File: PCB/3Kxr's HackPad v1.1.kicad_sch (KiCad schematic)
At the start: 8 parts, among them SW1 SW_Push, SW2 SW_Push, SW3 SW_Push, SW4 SW_Push, SW8 RotaryEncoder_Switch, U1 XIAO-RP2040-DIP

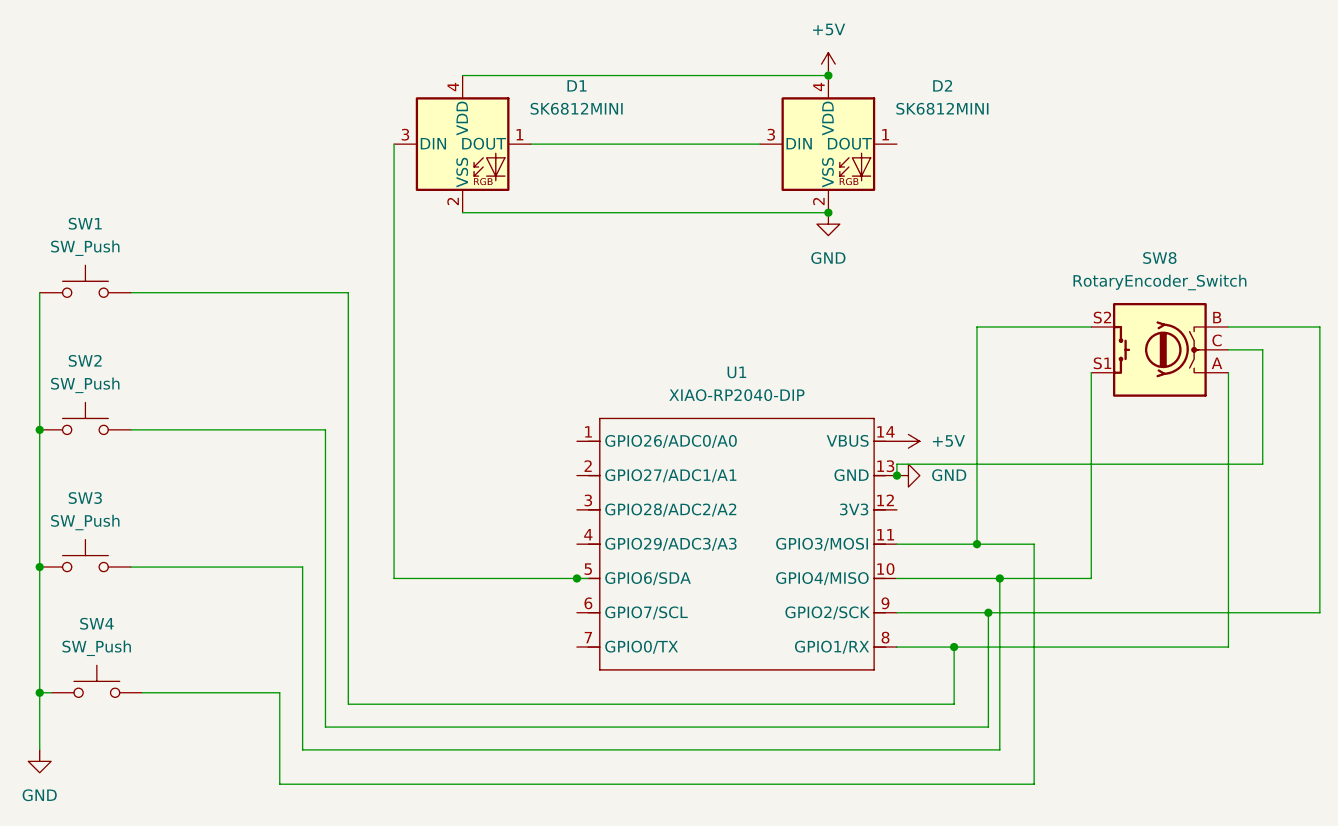
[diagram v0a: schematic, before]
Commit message: update HackPad v1.1
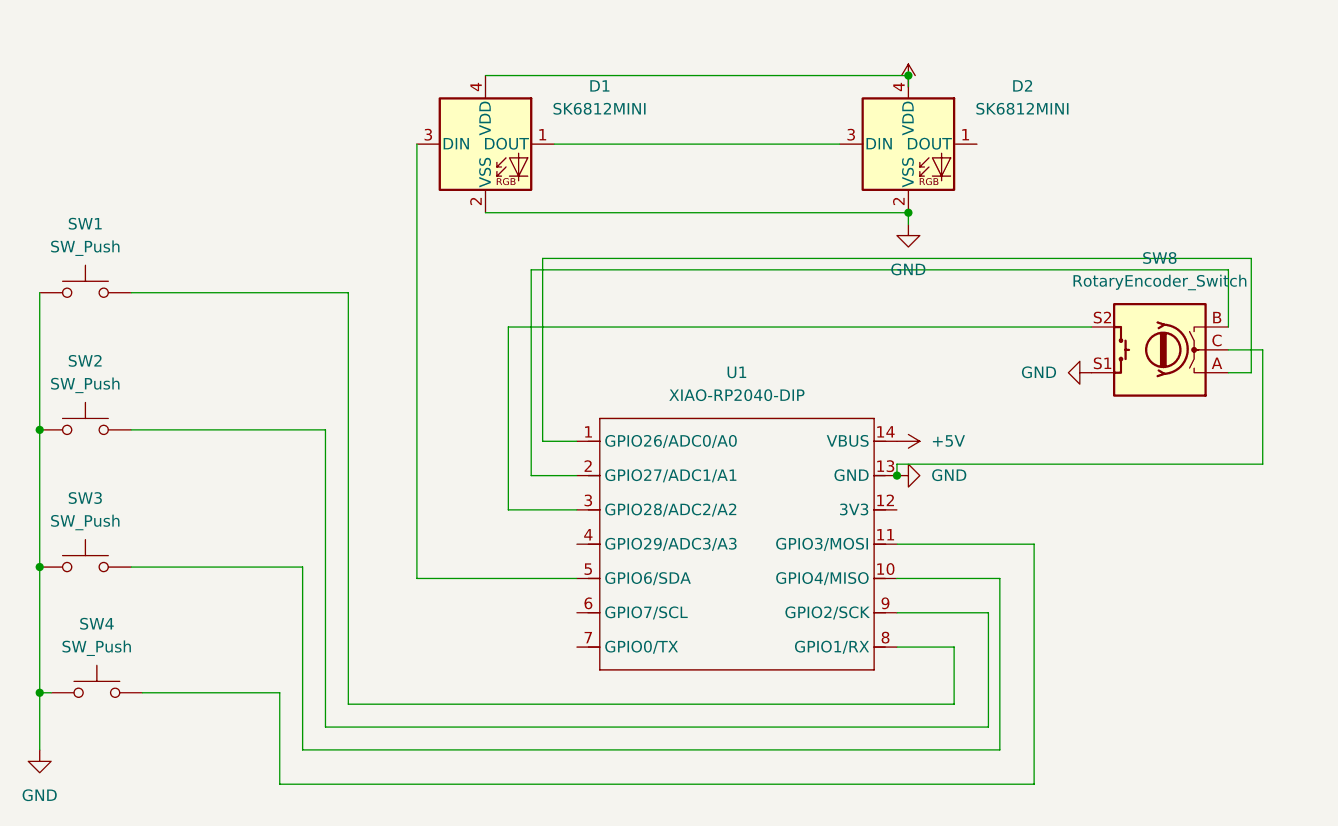
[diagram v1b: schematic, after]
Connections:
- net GND: now also SW8.S1
- net at U1.1 (GPIO26/ADC0/A0): now also SW8.A
- net at SW3.2, U1.10 (GPIO4/MISO): no longer SW8.S1
- net at SW4.2, U1.11 (GPIO3/MOSI): no longer SW8.S2
- net at U1.2 (GPIO27/ADC1/A1): now also SW8.B
- net at U1.3 (GPIO28/ADC2/A2): now also SW8.S2
- net at SW1.2, U1.8 (GPIO1/RX): no longer SW8.A
- net at SW2.2, U1.9 (GPIO2/SCK): no longer SW8.B
